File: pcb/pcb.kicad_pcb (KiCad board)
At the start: 2 copper layers, 60 x 60 mm, 13 parts, among them SW2 SW_Push

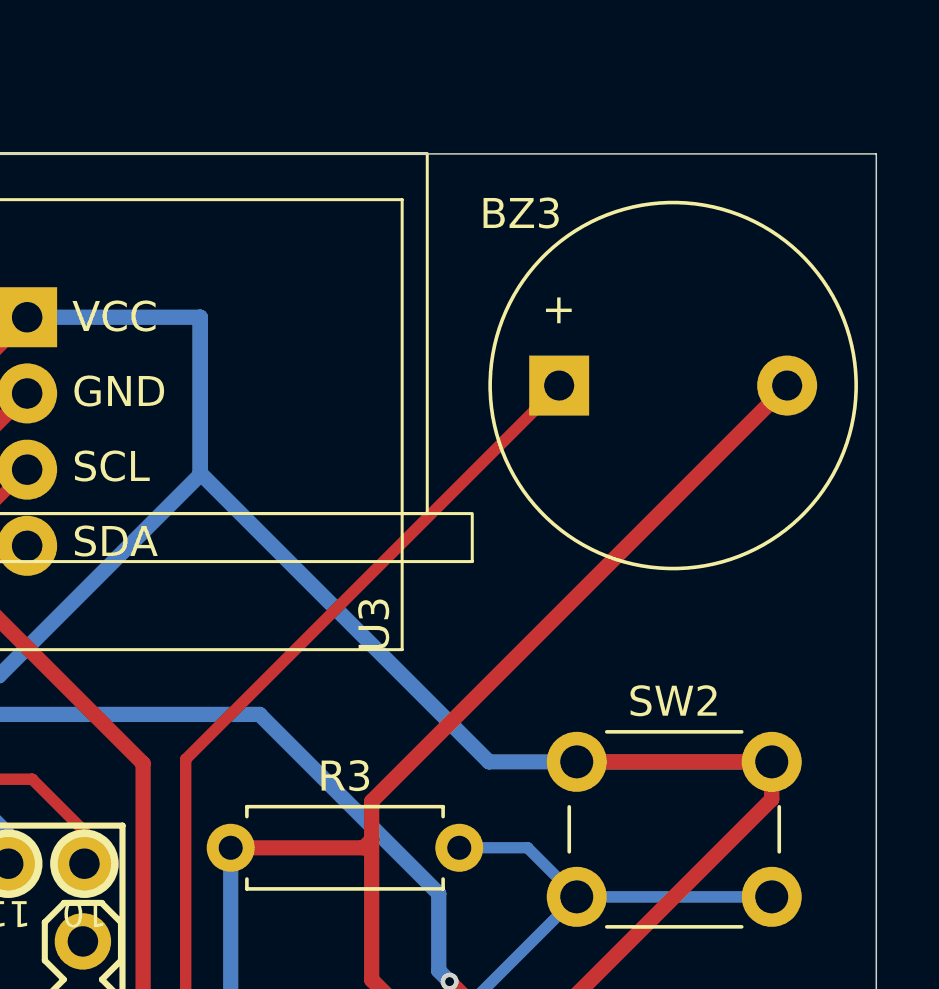
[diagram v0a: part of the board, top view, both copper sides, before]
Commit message: 5.16
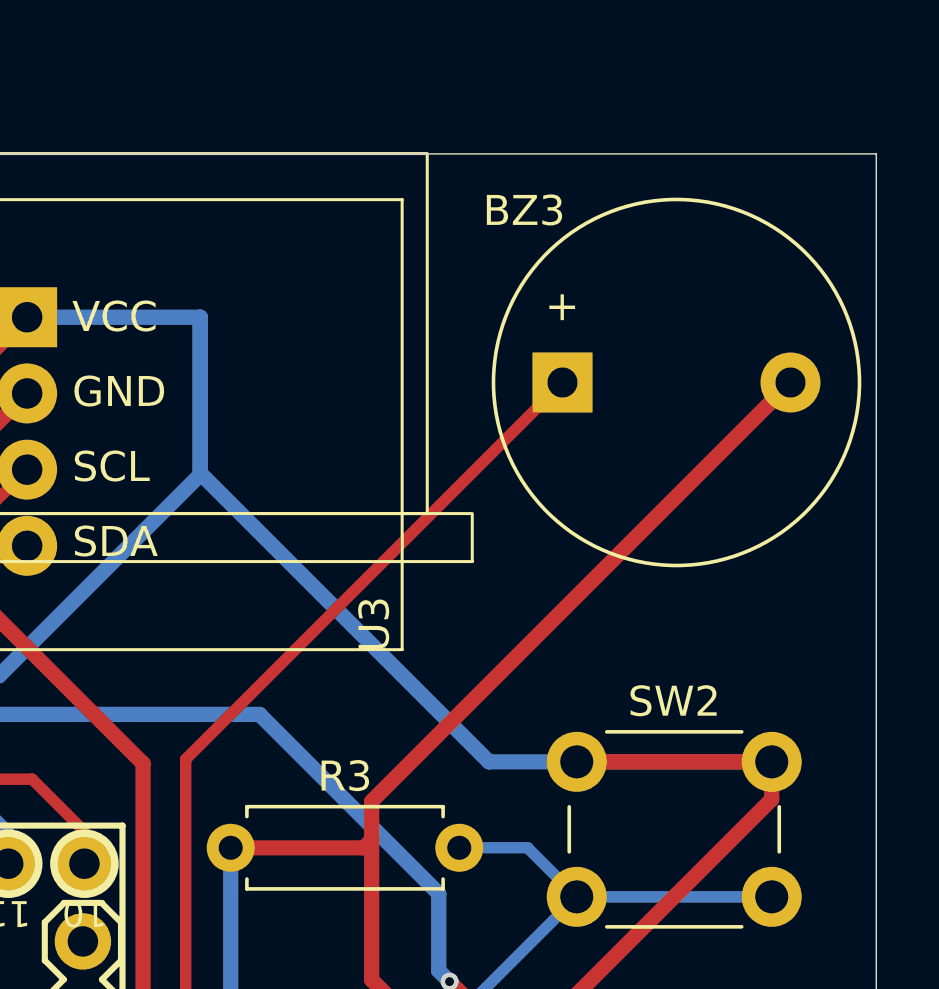
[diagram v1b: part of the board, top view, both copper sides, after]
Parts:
- moved BZ3 0.15 mm to (143.5, 76.2)
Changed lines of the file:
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@@
 	(footprint "Buzzer_Beeper:Buzzer_12x9.5RM7.6"
 		(layer "F.Cu")
-		(at 143.4084 76.3016)
+		(at 143.52 76.2)
 		(descr "Generic Buzzer, D12mm height 9.5mm with RM7.6mm")
 		(tags "buzzer")
@@
 		)
 	)
-	(dimension
-		(type orthogonal)
-		(layer "Edge.Cuts")
-		(pts
-			(xy 147.32 76.2) (xy 153.42 76.2)
-		)
-		(height -3.81)
-		(orientation 0)
-		(format
-			(prefix "")
-			(suffix "")
-			(units 3)
-			(units_format 0)
-			(precision 4)
-			(suppress_zeroes yes)
-		)
-		(style
-			(thickness 0.05)
-			(arrow_length 1.27)
-			(text_position_mode 0)
-			(arrow_direction outward)
-			(extension_height 0.58642)
-			(extension_offset 0.5)
-			(keep_text_aligned yes)
-		)
-		(gr_text "6.1"
-			(at 150.37 71.24 0)
-			(layer "Edge.Cuts")
-			(effects
-				(font
-					(size 1 1)
-					(thickness 0.15)
-				)
-			)
-		)
-	)
 	(via
 		(at 50.8 50.8)
@@
 	)
 	(segment
-		(start 151.0084 76.3116)
-		(end 151.0084 76.3016)
+		(start 137.16 90.16)
+		(end 151.12 76.2)
 		(width 0.508)
 		(layer "F.Cu")
@@
 	)
 	(segment
-		(start 137.16 90.16)
-		(end 151.0084 76.3116)
-		(width 0.508)
-		(layer "F.Cu")
-		(net 1)
-	)
-	(segment
 		(start 123.7996 83.1596)
 		(end 129.54 88.9)
@@
 	)
 	(segment
-		(start 137.16 91.44)
-		(end 137.16 90.16)
+		(start 129.54 97.9043)
+		(end 127.5334 99.9109)
 		(width 0.508)
 		(layer "F.Cu")
@@
 	)
 	(segment
-		(start 129.54 97.9043)
-		(end 127.5334 99.9109)
+		(start 137.16 91.44)
+		(end 137.16 90.16)
 		(width 0.508)
 		(layer "F.Cu")
@@
 	)
 	(segment
-		(start 143.4084 76.3016)
-		(end 143.4084 76.3116)
-		(width 0.381)
-		(layer "F.Cu")
-		(net 12)
-	)
-	(segment
-		(start 130.9605 100.2844)
-		(end 124.9426 106.3023)
+		(start 143.52 76.2)
+		(end 130.9605 88.7595)
 		(width 0.381)
 		(layer "F.Cu")
@@
 	)
 	(segment
-		(start 143.4084 76.3116)
-		(end 130.9605 88.7595)
+		(start 130.9605 100.2844)
+		(end 124.9426 106.3023)
 		(width 0.381)
 		(layer "F.Cu")
